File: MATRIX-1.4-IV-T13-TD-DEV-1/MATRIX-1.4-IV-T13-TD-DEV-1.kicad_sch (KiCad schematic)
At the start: 186 parts, among them Q401 MPSA42, Q402 MPSA42, Q403 MJE340, Q404 MJE350, Q405 MJE350, Q406 MJE350, Q407 MJE340, Q408 MJE350, Q409 MJE340, Q410 MJE15032, Q411 MJE15033, Q412 2SC5200, Q413 2SA1943, Q4141 2SC5200, Q41410 2SC5200, Q4142 2SC5200, Q4143 2SC5200, Q4144 2SC5200, Q4145 2SC5200, Q4146 2SC5200, Q4147 2SC5200, Q4148 2SC5200, Q4149 2SC5200, Q4151 2SA1943, Q41510 2SA1943, Q4152 2SA1943, Q4153 2SA1943, Q4154 2SA1943, Q4155 2SA1943, Q4156 2SA1943, Q4157 2SA1943, Q4158 2SA1943, Q4159 2SA1943, Q601 MJE340, Q602 MJE15032, Q603 2SC5200, Q604 2N5551, Q605 2N5401, Q606 2N5401, Q607 MJE340, Q608 2N5401, Q609 2N5401, Q701 MJE350, Q702 MJE15033, Q703 2SA1943, Q704 2N5401, Q705 2N5551, Q706 2N5551, Q707 MJE350, Q708 2N5551, Q709 2N5551

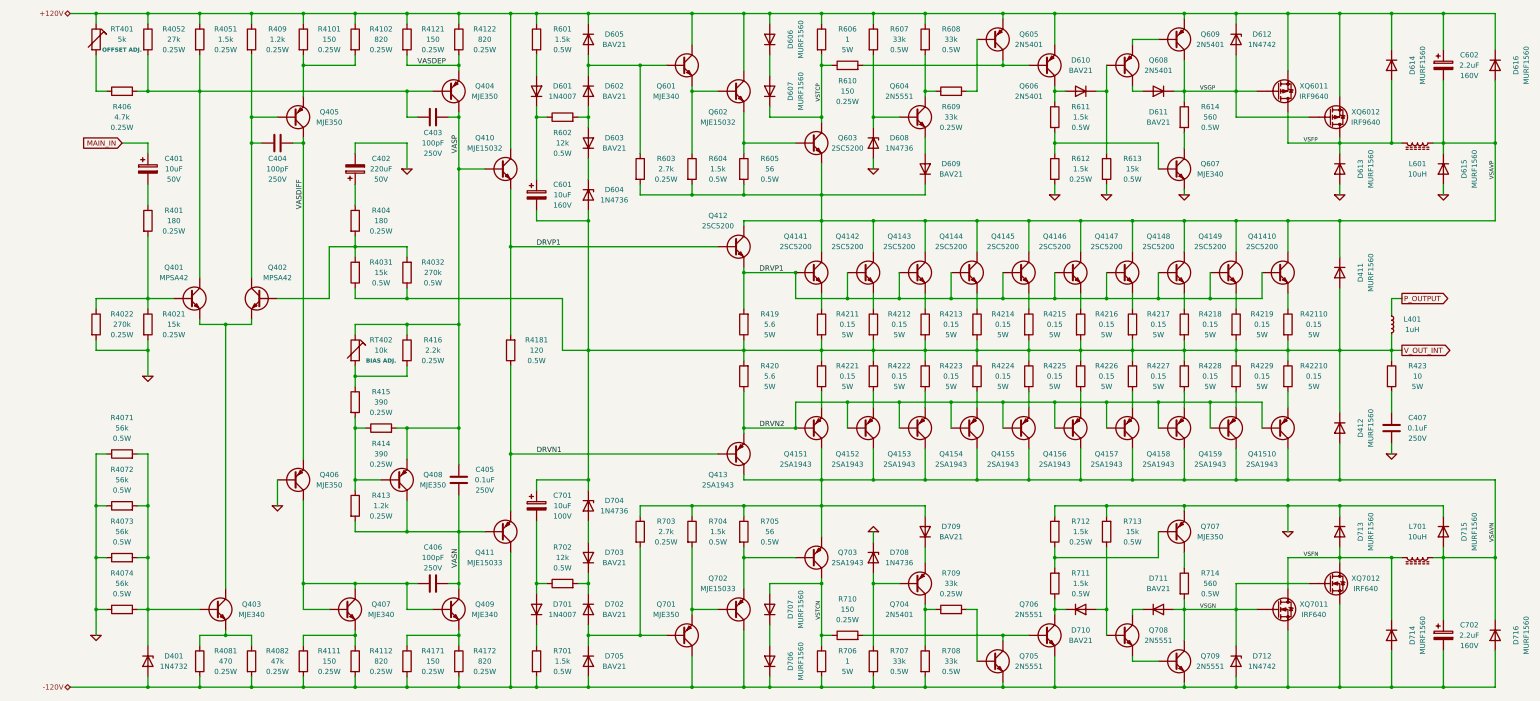
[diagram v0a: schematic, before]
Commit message: Routine Update Sun Jul 10 09:42:39 PM WIB 2022
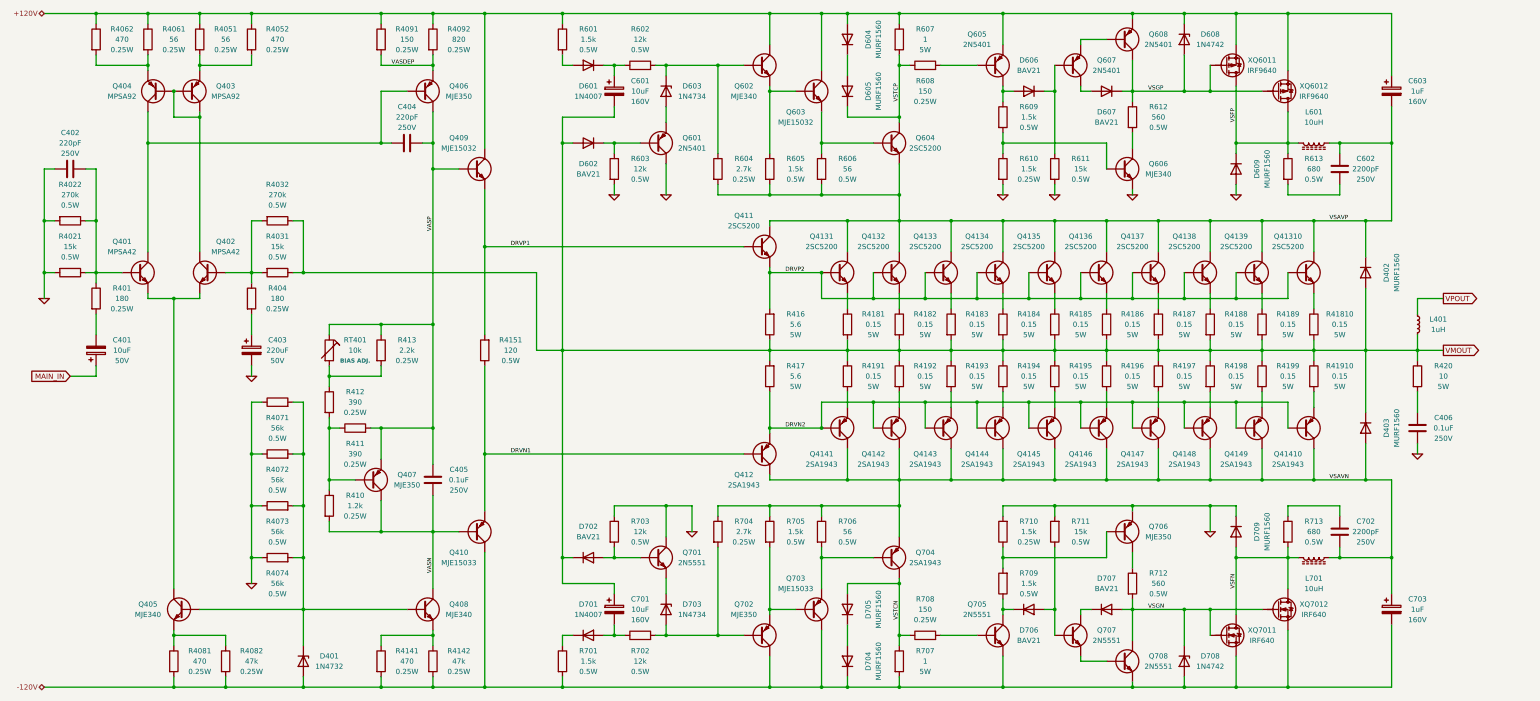
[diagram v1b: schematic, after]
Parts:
- removed C404, C406: 100pF, MATRIX_1.4:CAPACITOR_CERAMIC_STD, symbol Device:C
- removed D603, D605, D609, D703, D705, D709: BAV21, MATRIX_1.4:DIODE_AXIAL_SMALL_SI, symbol MATRIX_1.4:D
- removed D604, D608, D704, D708: 1N4736, MATRIX_1.4:DIODE_AXIAL_SMALL_SI, symbol MATRIX_1.4:D_Zener
- removed D614, D615, D616, D714, D715, D716: MURF1560, MATRIX_1.4:DIODE_AXIAL_SMALL_GE, symbol MATRIX_1.4:D
- removed Q405, Q406: MJE350, MATRIX_1.4:TO-225, symbol MATRIX_1.4:Q_PNP_CBE
- removed Q407: MJE340, MATRIX_1.4:TO-225, symbol MATRIX_1.4:Q_NPN_CBE
- removed Q604, Q705: 2N5551, MATRIX_1.4:TO-92-EBC, symbol MATRIX_1.4:Q_NPN_CBE
- removed Q605, Q704: 2N5401, MATRIX_1.4:TO-92-EBC, symbol MATRIX_1.4:Q_PNP_CBE
- removed R406: 4.7k, MATRIX_1.4:RESISTOR_AXIAL_0.25W, symbol Device:R
- removed R409: 1.2k, MATRIX_1.4:RESISTOR_AXIAL_0.25W, symbol Device:R
- removed R4101, R4111: 150, MATRIX_1.4:RESISTOR_AXIAL_0.25W, symbol Device:R
- removed R4102, R4112: 820, MATRIX_1.4:RESISTOR_AXIAL_0.25W, symbol Device:R
- removed R607, R608, R707, R708: 33k, MATRIX_1.4:RESISTOR_AXIAL_0.5W, symbol Device:R
- removed R609, R709: 33k, MATRIX_1.4:RESISTOR_AXIAL_0.25W, symbol Device:R
- removed RT401: 2.5k, MATRIX_1.4:RESISTOR_ROUND_TRIMPOT_STD, symbol Device:R_Trim
- added C402: 220pF, MATRIX_1.4:CAPACITOR_CERAMIC_STD, symbol Device:C
- added C602, C702: 2200pF, MATRIX_1.4:CAPACITOR_MPF_STD, symbol Device:C
- added D603, D703: 1N4734, MATRIX_1.4:DIODE_AXIAL_SMALL_SI, symbol MATRIX_1.4:D_Zener
- added Q403, Q404: MPSA92, MATRIX_1.4:TO-92-EBC, symbol MATRIX_1.4:Q_PNP_CBE
- added Q601: 2N5401, MATRIX_1.4:TO-92-EBC, symbol MATRIX_1.4:Q_PNP_CBE
- added Q701: 2N5551, MATRIX_1.4:TO-92-EBC, symbol MATRIX_1.4:Q_NPN_CBE
- added R4061: 56, MATRIX_1.4:RESISTOR_AXIAL_0.25W, symbol Device:R
- added R4062: 470, MATRIX_1.4:RESISTOR_AXIAL_0.25W, symbol Device:R
- added R603, R703: 12k, MATRIX_1.4:RESISTOR_AXIAL_0.5W, symbol Device:R
- added R613, R713: 680, MATRIX_1.4:RESISTOR_AXIAL_0.5W, symbol Device:R
- C404: renamed from C403; value 100pF -> 220pF
- C603: renamed from C602; value 2.2uF -> 1uF
- C701: Voltage 100V -> 160V
- C703: renamed from C702; value 2.2uF -> 1uF
- D602: Spice_Model BAV21 -> 1N4007
- R4021, R4022: footprint MATRIX_1.4:RESISTOR_AXIAL_0.25W -> MATRIX_1.4:RESISTOR_AXIAL_0.5W; Wattage 0.25W -> 0.5W
- R4051: value 1.5k -> 56
- R4052: value 27k -> 470
- R4141: renamed from R4171; value 150 -> 470
- R4142: renamed from R4172; value 820 -> 47k
- XQ6011, XQ6012: symbol Device:Q_PMOS_DGS -> MATRIX_1.4:Q_PMOS_DGS
- XQ7011, XQ7012: symbol Device:Q_NMOS_DGS -> MATRIX_1.4:Q_NMOS_DGS
- renumbered C402 to C403, C407 to C406, D411 to D402, D412 to D403, D606 to D604, D607 to D605, D610 to D606, D611 to D607, D612 to D608, D613 to D609, D706 to D704, D707 to D705, D710 to D706, D711 to D707, D712 to D708, D713 to D709, Q403 to Q405, Q404 to Q406, Q408 to Q407, Q409 to Q408, Q410 to Q409, Q411 to Q410, Q412 to Q411, Q413 to Q412, Q4141 to Q4131, Q41410 to Q41310, Q4142 to Q4132, Q4143 to Q4133, Q4144 to Q4134, Q4145 to Q4135, Q4146 to Q4136, Q4147 to Q4137, Q4148 to Q4138, Q4149 to Q4139, Q4151 to Q4141, Q41510 to Q41410, Q4152 to Q4142, Q4153 to Q4143, Q4154 to Q4144, Q4155 to Q4145, Q4156 to Q4146, Q4157 to Q4147, Q4158 to Q4148, Q4159 to Q4149, Q601 to Q602, Q602 to Q603, Q603 to Q604, Q606 to Q605, Q607 to Q606, Q608 to Q607, Q609 to Q608, Q701 to Q702, Q702 to Q703, Q703 to Q704, Q706 to Q705, Q707 to Q706, Q708 to Q707, Q709 to Q708, R4121 to R4091, R4122 to R4092, R413 to R410, R414 to R411, R415 to R412, R416 to R413, R4181 to R4151, R419 to R416, R420 to R417, R4211 to R4181, R42110 to R41810, R4212 to R4182, R4213 to R4183, R4214 to R4184, R4215 to R4185, R4216 to R4186, R4217 to R4187, R4218 to R4188, R4219 to R4189, R4221 to R4191, R42210 to R41910, R4222 to R4192, R4223 to R4193, R4224 to R4194, R4225 to R4195, R4226 to R4196, R4227 to R4197, R4228 to R4198, R4229 to R4199, R423 to R420, R603 to R604, R604 to R605, R605 to R606, R606 to R607, R610 to R608, R611 to R609, R612 to R610, R613 to R611, R614 to R612, R703 to R704, R704 to R705, R705 to R706, R706 to R707, R710 to R708, R711 to R709, R712 to R710, R713 to R711, R714 to R712, RT402 to RT401
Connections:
- net V_OUT_INT is gone; now on net VMOUT: C601.2, C701.1, D402.1 (A), D403.2 (K), L401.2, R4031.1, R4032.1, R416.1, R417.2, R4181.2, R41810.2, R4182.2, R4183.2, R4184.2, R4185.2, R4186.2, R4187.2, R4188.2, R4189.2, R4191.1, R41910.1, R4192.1, R4193.1, R4194.1, R4195.1, R4196.1, R4197.1, R4198.1, R4199.1, R420.1
- net +120V: now also R4061.1, R4062.1
- net 0: now also C402.1, Q601.1 (C), Q701.1 (C), R603.2, R703.1
- net DRVP1: no longer Q411.3 (E), Q4131.2 (B), Q41310.2 (B), Q4132.2 (B), Q4133.2 (B), Q4134.2 (B), Q4135.2 (B), Q4136.2 (B), Q4137.2 (B), Q4138.2 (B), Q4139.2 (B), R416.2
- net VSAVN: now also C702.1
- net VSAVP: now also C602.2
- net VSFN: now also R713.2
- net VSFP: now also R613.1
- net at Q702.2 (B), R704.2: now also R702.2, D703.1 (A); no longer D702.1 (A)
- net VMOUT: now reaches D702.2 (K)
- net VMOUT: now also D602.1 (A); no longer R702.2
- net at C401.2: now also R401.2; no longer R401.1
- net at Q401.2 (B), R4021.1, R4022.1: now also R401.1, C402.2; no longer R401.2
- net at D401.2 (K), Q405.2 (B), R4071.2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: now also Q408.2 (B)
- net at C404.1, Q401.1 (C), Q406.2 (B): now also Q404.1 (C); no longer R4051.2, R4052.2
- net at R602.2: now also Q602.2 (B), R604.1, D603.2 (K); no longer D602.1 (A)
- net at Q402.1 (C): now also Q403.1 (C), Q403.2 (B), Q404.2 (B)
- net at R404.1: now also Q402.2 (B), R4031.2, R4032.2; no longer C403.1
- net P_OUTPUT renamed VPOUT
- new net: D602.2 (K), Q601.2 (B), R603.1
- new net: Q404.3 (E), R4061.2, R4062.2
- new net: C702.2, R713.1
- new net: Q403.3 (E), R4051.2, R4052.2
- new net: D702.1 (A), Q701.2 (B), R703.2
- new net: D703.2 (K), Q701.3 (E)
- new net: C403.1, R404.2
- new net: D603.1 (A), Q601.3 (E)
- new net: C602.1, R613.2
- new net DRVP2: Q411.3 (E), Q4131.2 (B), Q41310.2 (B), Q4132.2 (B), Q4133.2 (B), Q4134.2 (B), Q4135.2 (B), Q4136.2 (B), Q4137.2 (B), Q4138.2 (B), Q4139.2 (B), R416.2
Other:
- title: 1400 WATTS RMS CLASS H\nAUDIO POWER AMPLIFIER\nFOR 4-OHMS LOUDSPEAKER -> 1400 WATTS RMS CLASS-TD\nAUDIO POWER AMPLIFIER\nFOR 4-OHMS LOUDSPEAKER
- moved on the sheet: C401, C403, C404, C405, C406, C601, C603, C703, D402, D403, D604, D605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
